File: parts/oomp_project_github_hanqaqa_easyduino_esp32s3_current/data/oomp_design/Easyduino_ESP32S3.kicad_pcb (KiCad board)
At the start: 4 copper layers, 25.9 x 63.9 mm, 35 parts, among them J1 USB_C_Receptacle_USB2.0, J2 USB_C_Receptacle_USB2.0, Q1 Q_NPN_BCE, Q2 Q_NPN_BCE, SW1 SW_Push, SW2 SW_Push, U1 ESP32-S3-WROOM-1, U2 ESP32-S3-DevKitC, U3 CP2102N-Axx-xQFN28, U5 AMS1117-3.3

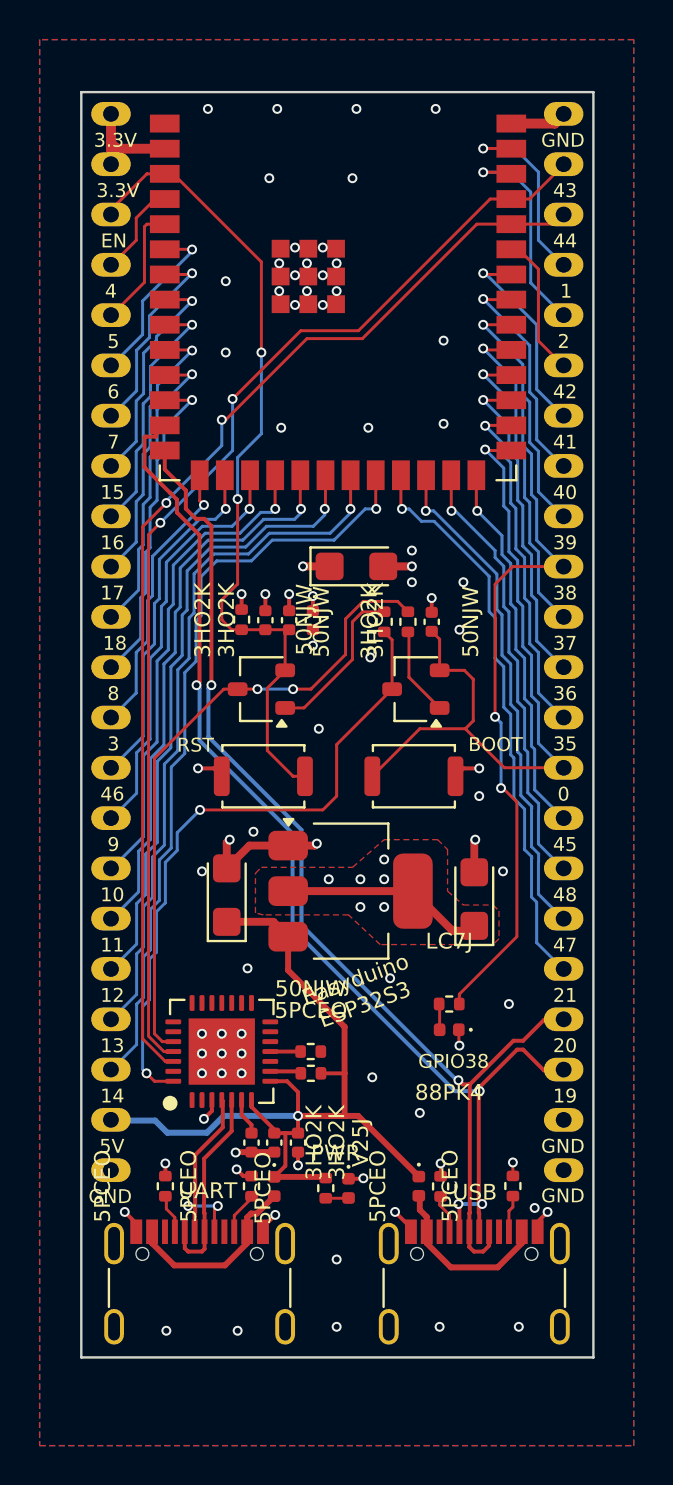
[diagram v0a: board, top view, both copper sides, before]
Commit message: working
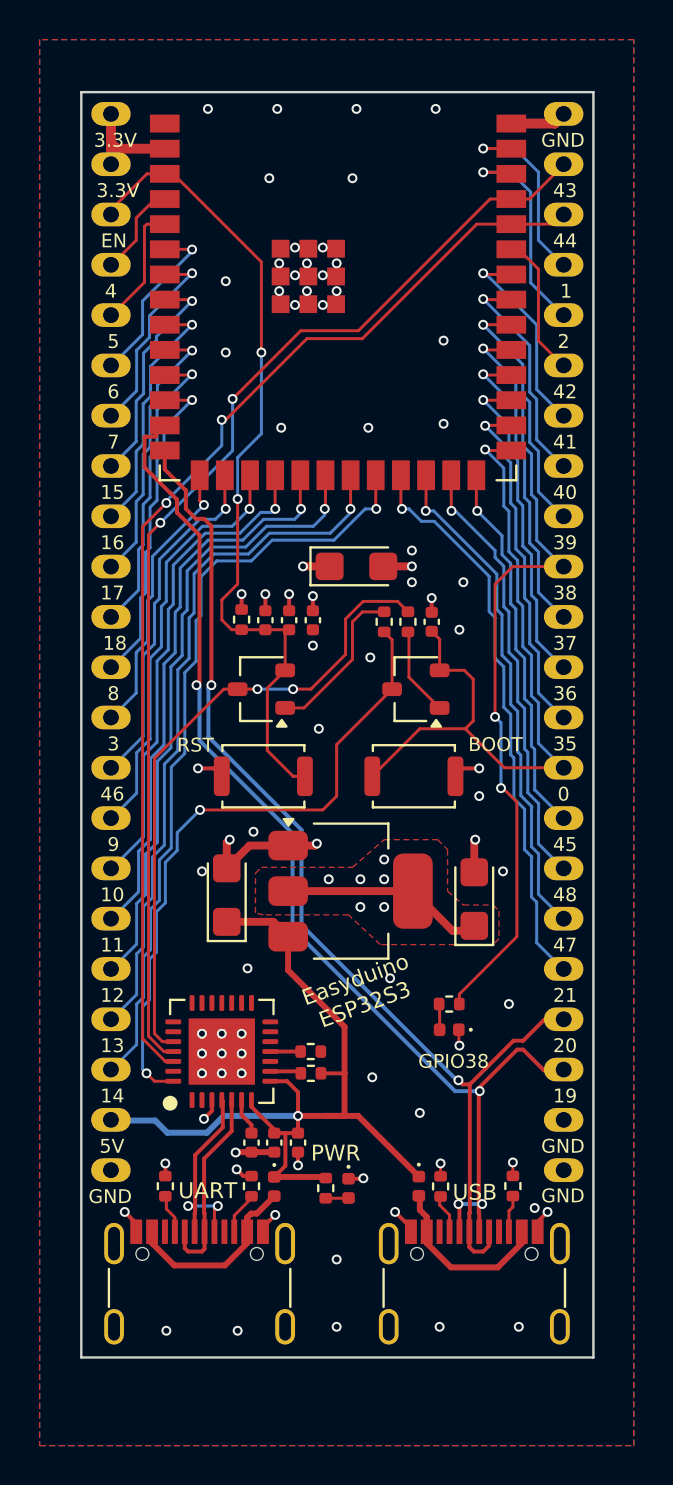
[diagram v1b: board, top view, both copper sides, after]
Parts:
- C1: footprint OOMP_MachineSolder:electronic_capacitor_0402_1_micro_farad -> Capacitor_SMD:C_0402_1005Metric
- C2, C3, C4, C5, C8, C9: footprint OOMP_MachineSolder:electronic_capacitor_0402_100_nano_farad -> Capacitor_SMD:C_0402_1005Metric
- D4: footprint OOMP_MachineSolder:electronic_led_0402 -> LED_SMD:LED_0402_1005Metric
- R1, R10, R4, R5: footprint OOMP_MachineSolder:electronic_resistor_0402_10000_ohm -> Resistor_SMD:R_0402_1005Metric
- R11, R2, R3, R6, R7, R8: footprint OOMP_MachineSolder:electronic_resistor_0402_5100_ohm -> Resistor_SMD:R_0402_1005Metric
- R9: footprint OOMP_MachineSolder:electronic_resistor_0402_2400_ohm -> Resistor_SMD:R_0402_1005Metric
